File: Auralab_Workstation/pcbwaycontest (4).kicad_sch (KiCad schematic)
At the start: 14 parts, among them J1 Conn_Coaxial, J2 TEST_SOCKET, Q1 BS170, SW1 SW_SPDT, U1 TL072, U2 MCP3201, U3 REF3033, U4 INA226

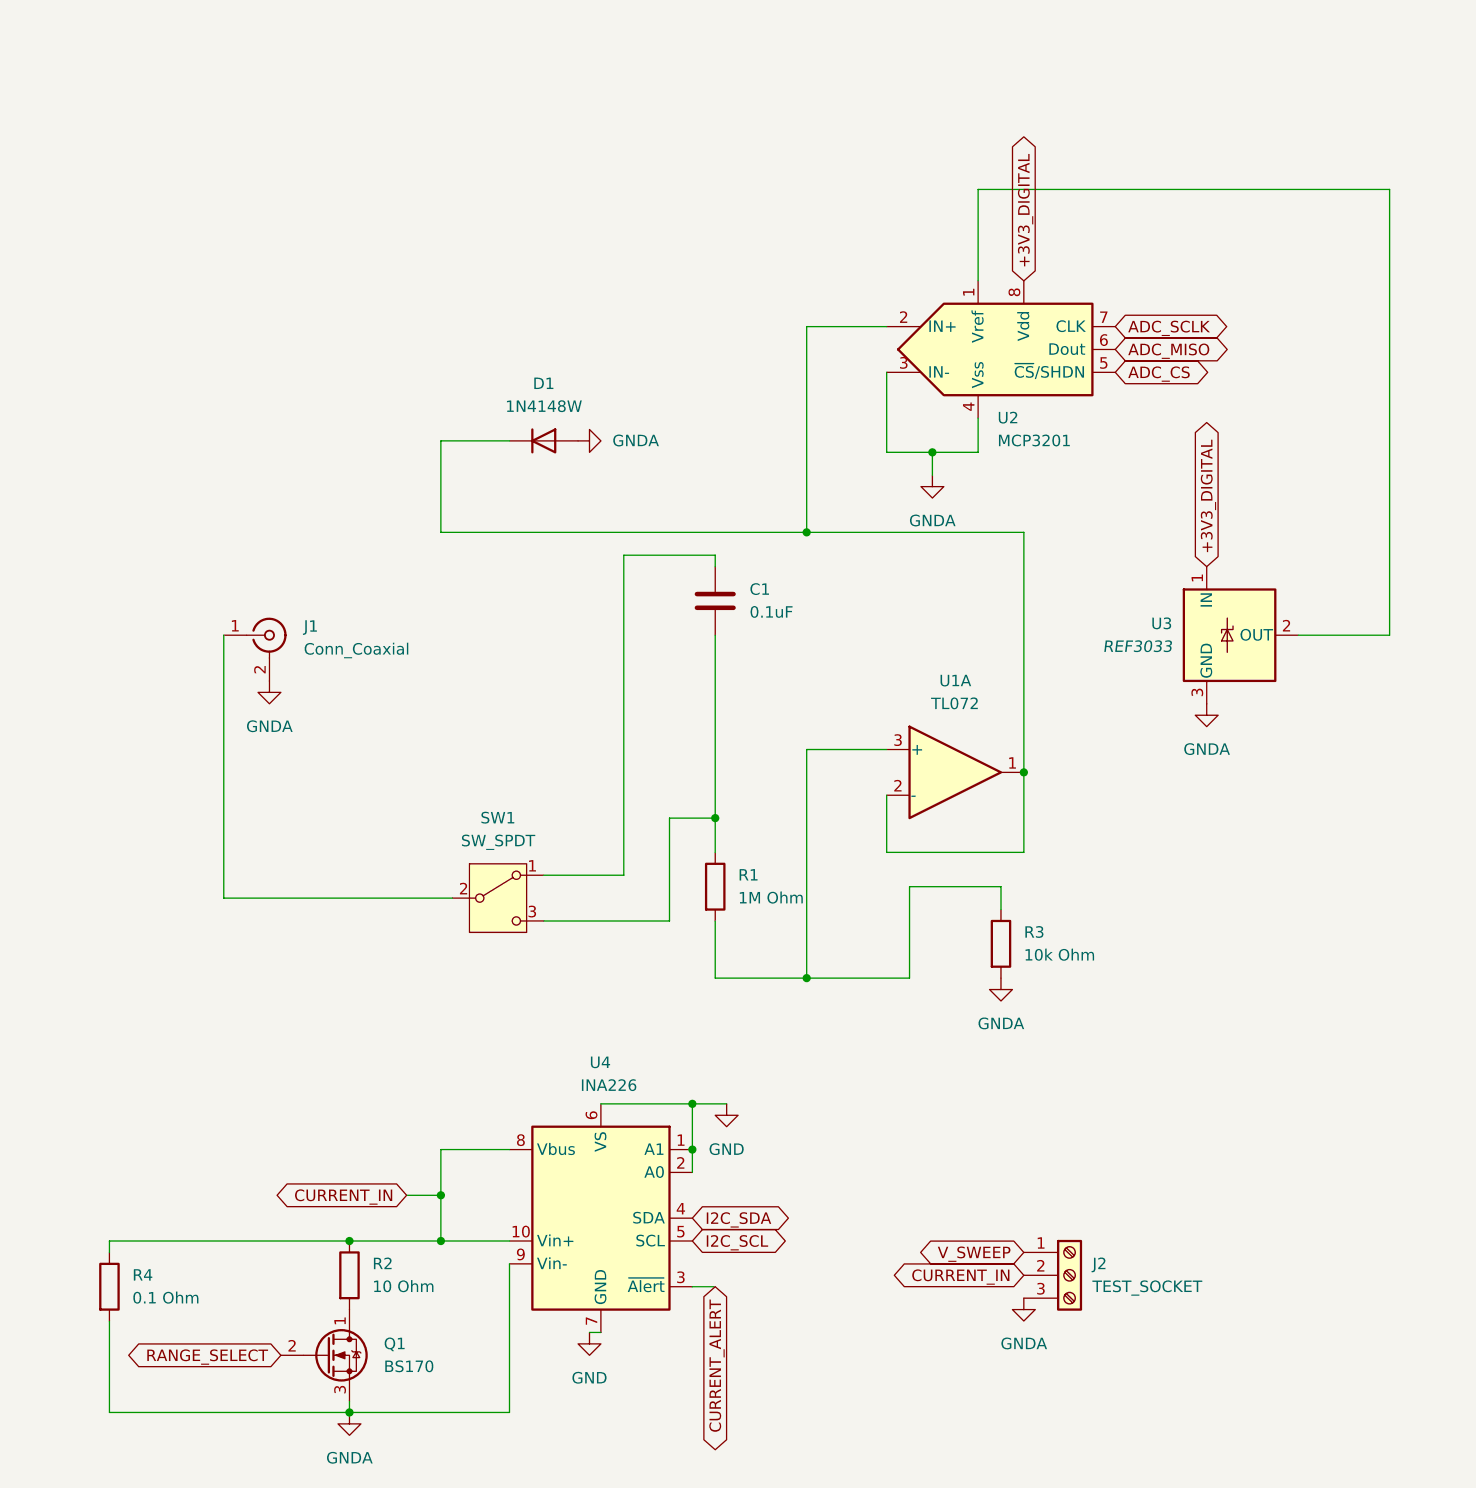
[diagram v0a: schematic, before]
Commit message: Check analog part
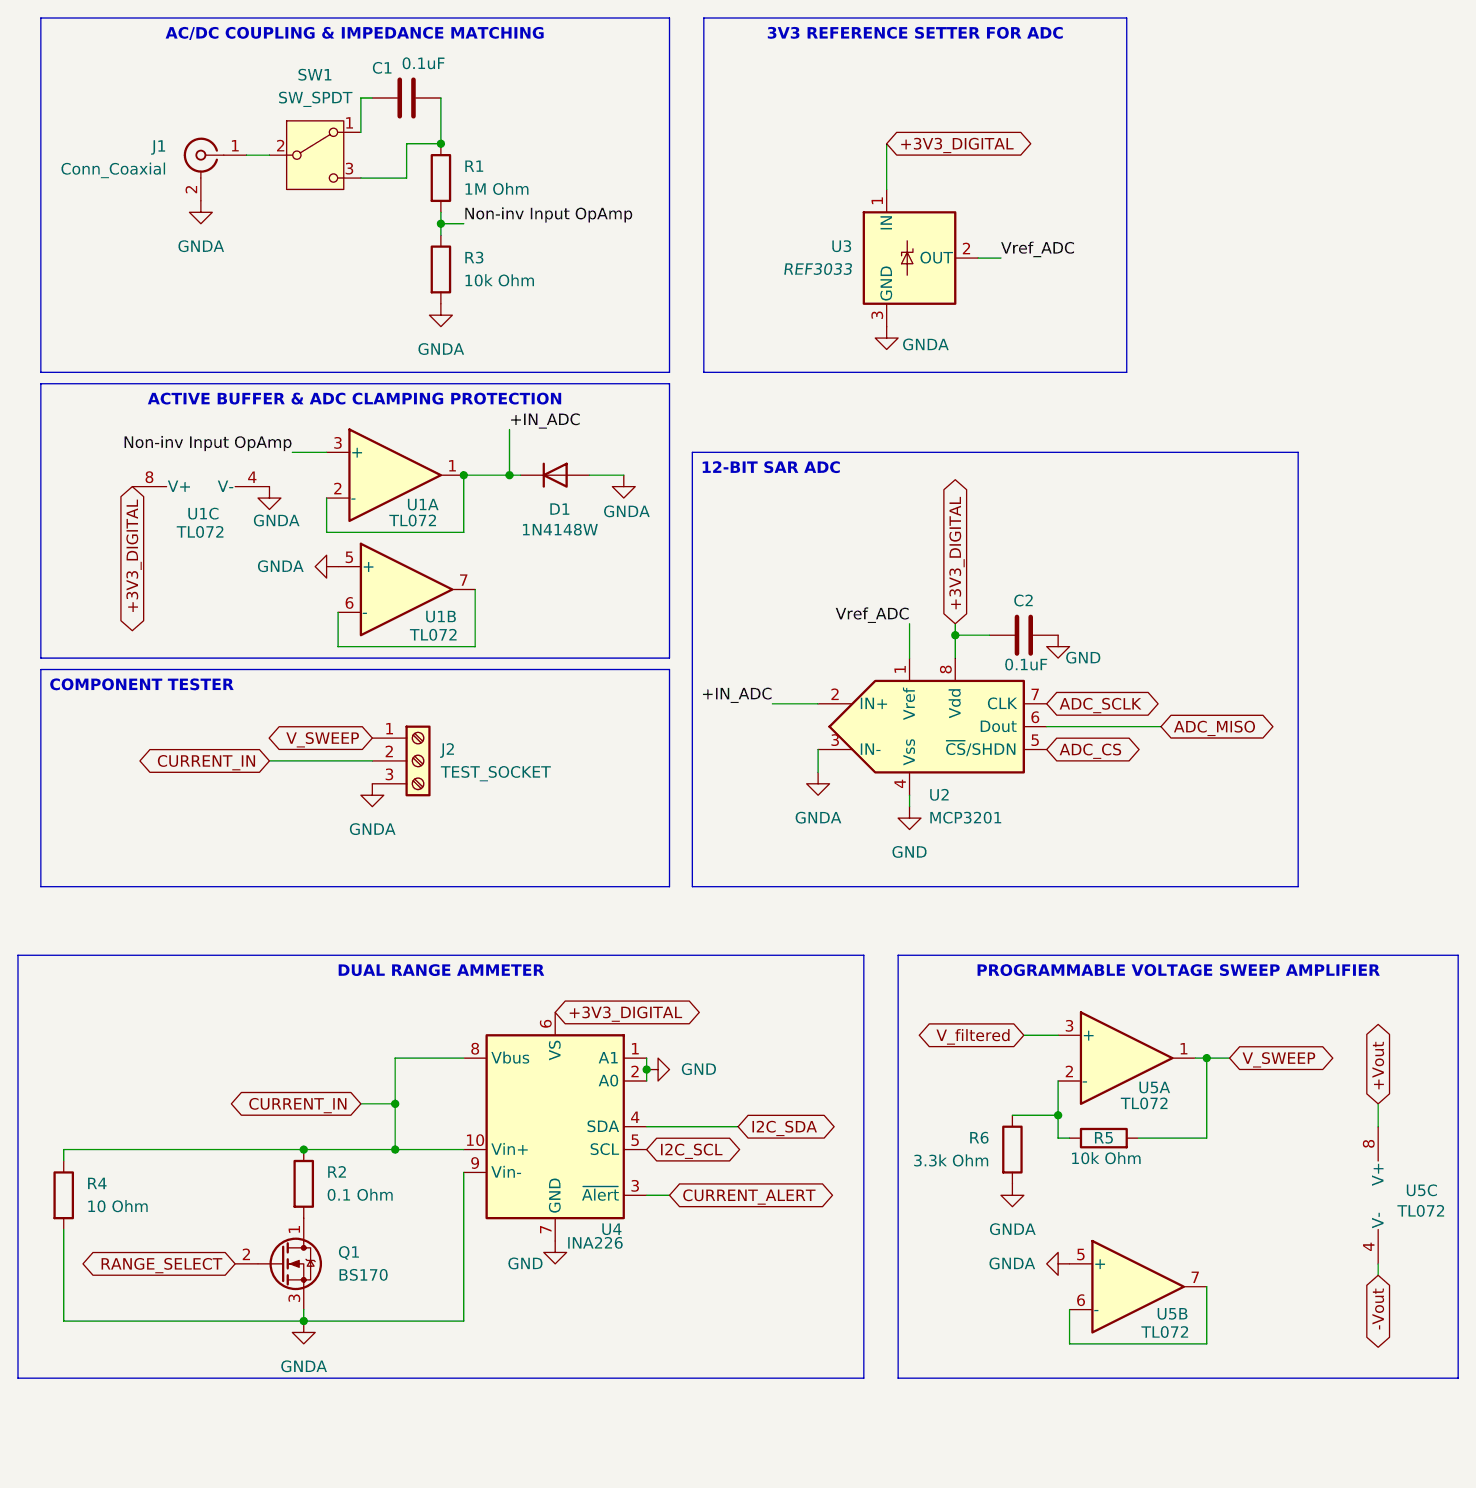
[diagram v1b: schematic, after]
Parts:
- added C2: 0.1uF, Capacitor_SMD:C_0805_2012Metric, symbol Device:C
- added R5: 10k Ohm, Resistor_SMD:R_0805_2012Metric, symbol Device:R
- added R6: 3.3k Ohm, Resistor_SMD:R_0805_2012Metric, symbol Device:R
- added unit 2 of U1
- added unit 3 of U1
- added U5: TL072, Package_SO:SOIC-8_3.9x4.9mm_P1.27mm, symbol Amplifier_Operational:TL072
- R2: value 10 Ohm -> 0.1 Ohm
- R4: value 0.1 Ohm -> 10 Ohm
- SW1: footprint Connector:FanPinHeader_1x03_P2.54mm_Vertical -> Button_Switch_SMD:SW_SPDT_PCM12
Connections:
- net +3V3_DIGITAL: now also U4.6 (VS), C2.1, U1.8 (V+)
- net GND: now also U2.4 (Vss), C2.2; no longer U4.6 (VS)
- net GNDA: now also R6.2, U1.4 (V-), U1.5 (+), U5.5 (+); no longer U2.4 (Vss)
- net V_SWEEP: now also R5.2, U5.1
- net Vref_ADC: now reaches U2.1 (Vref), U3.2 (OUT)
- net +IN_ADC: now reaches D1.1 (K), U1.1, U1.2 (-), U2.2 (IN+)
- net Non-inv Input OpAmp: now reaches R1.2, R3.1, U1.3 (+)
- new net: R5.1, R6.1, U5.2 (-)
- new net: U5.6 (-), U5.7
- new net: U1.6 (-), U1.7
- new net +Vout: U5.8 (V+)
- new net -Vout: U5.4 (V-)
- new net V_filtered: U5.3 (+)
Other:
- moved on the sheet: C1, D1, J1, J2, Q1, R1, R2, R3, R4, SW1, U1A, U2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
